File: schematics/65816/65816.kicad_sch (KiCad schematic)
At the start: 2 parts

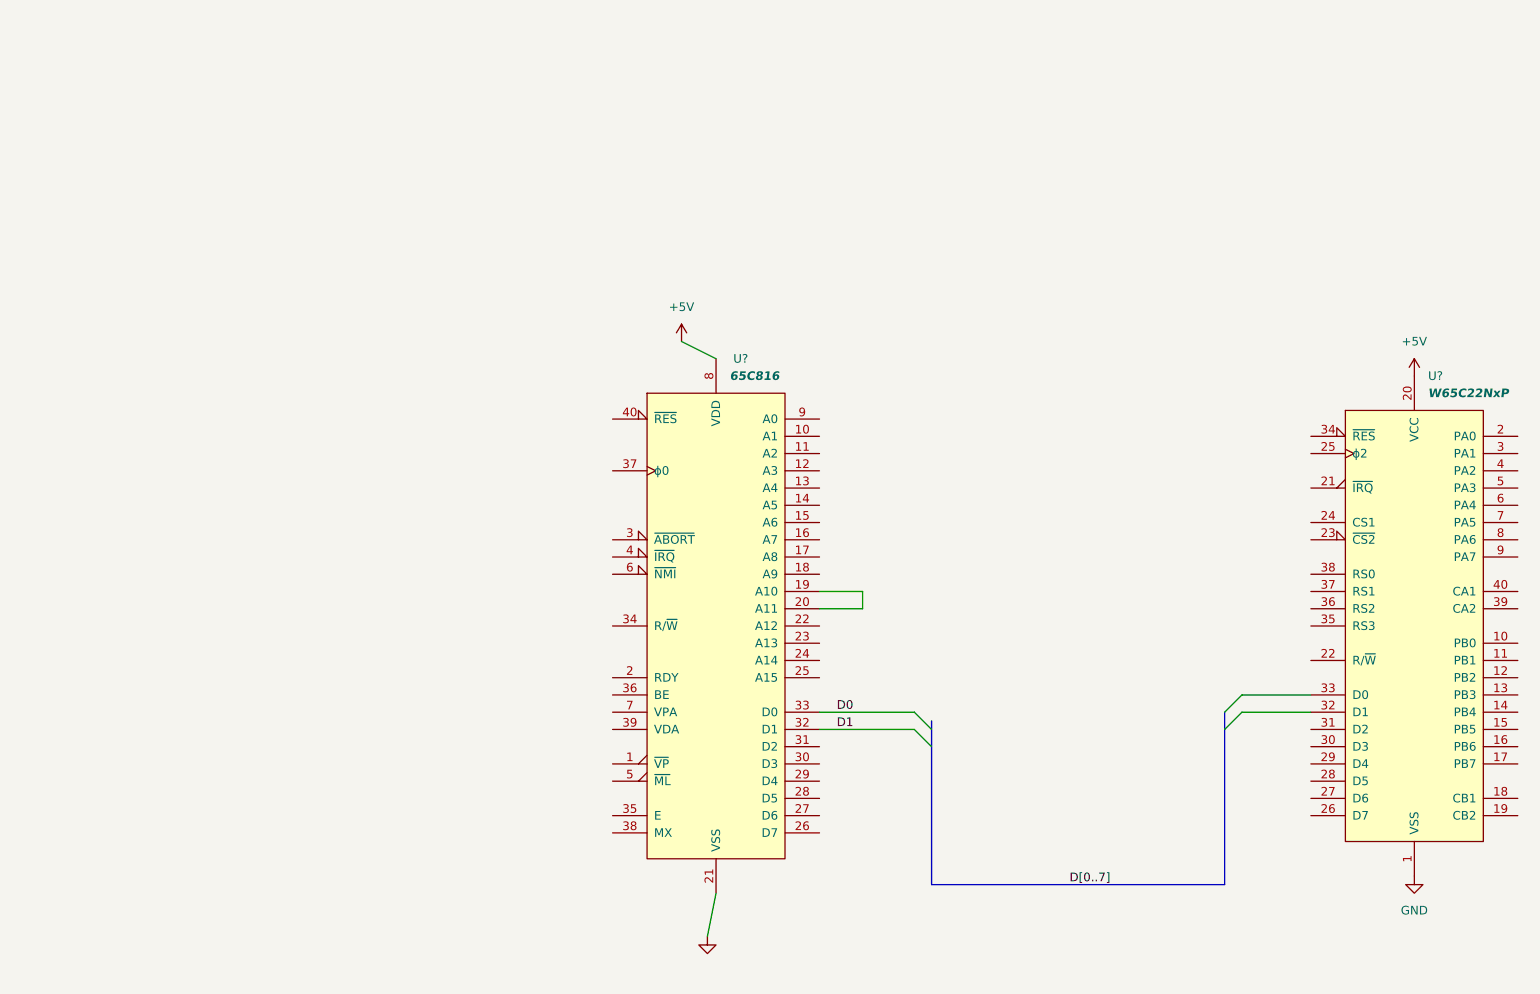
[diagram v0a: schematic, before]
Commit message: schematics
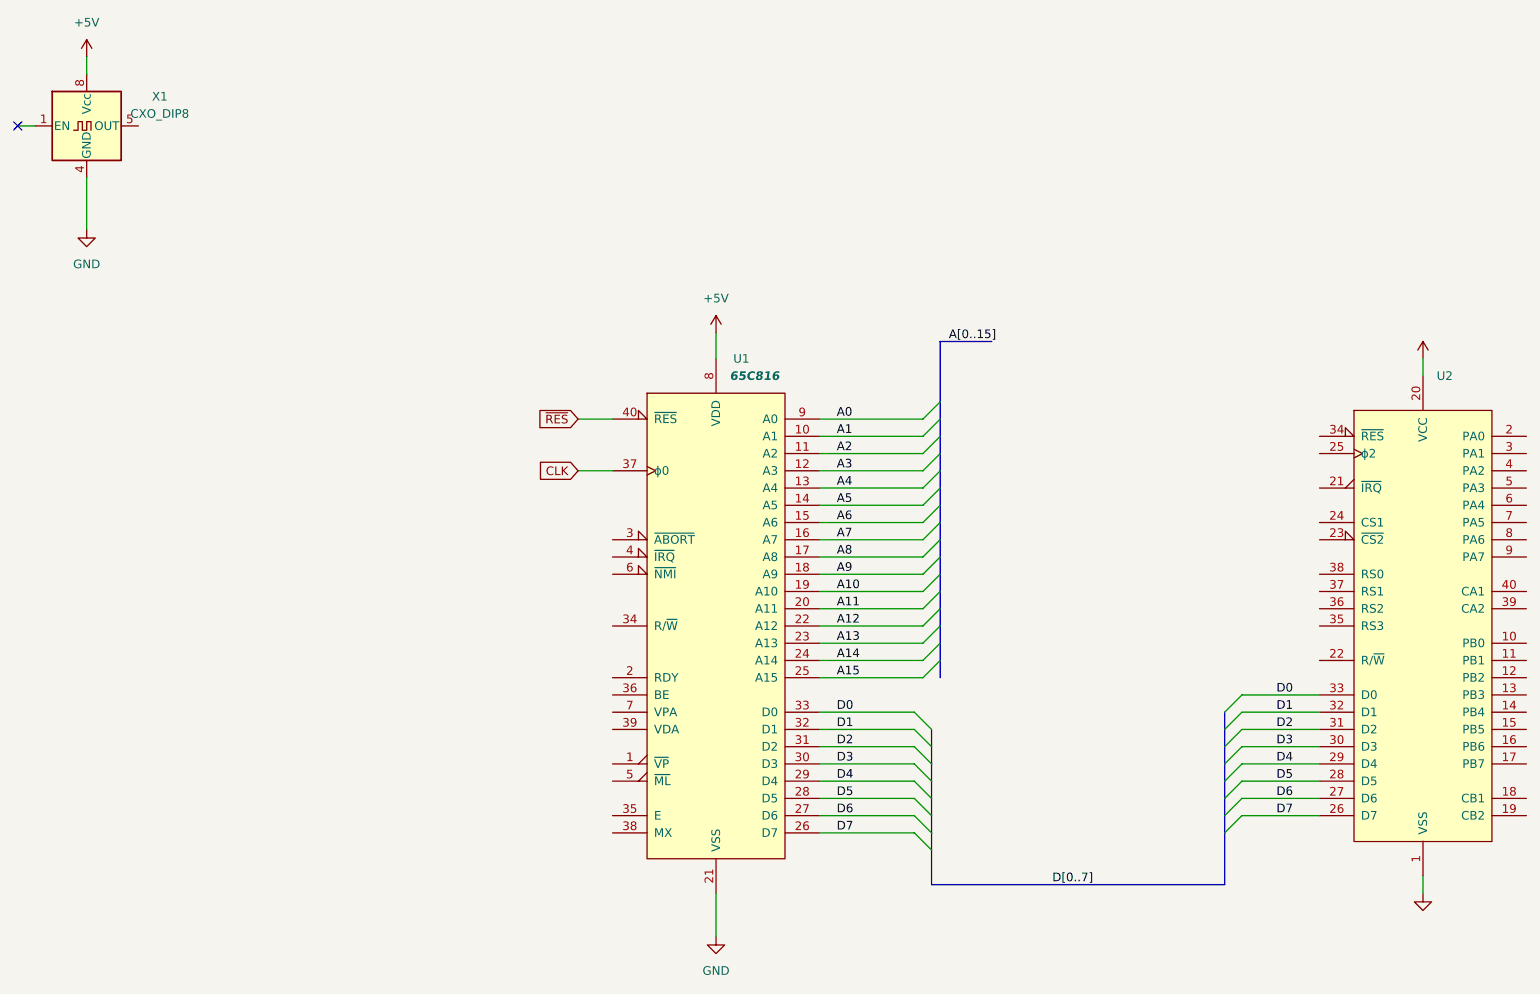
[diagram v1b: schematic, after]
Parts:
- added X1: CXO_DIP8, Oscillator:Oscillator_DIP-8, symbol Oscillator:CXO_DIP8
- U2: renamed from U?; value W65C22NxP -> (none)
- gave numbers to parts that had none: 1
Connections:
- net +5V: now also X1.8 (Vcc)
- net D0: now also U2.33 (D0)
- net D1: now also U2.32 (D1)
- net GND: now also X1.4 (GND)
- net D7: now reaches U2.26 (D7)
- net D7: now also U1.26 (D7)
- net D6: now reaches U2.27 (D6)
- net D6: now also U1.27 (D6)
- net D5: now reaches U2.28 (D5)
- net D5: now also U1.28 (D5)
- net D4: now reaches U2.29 (D4)
- net D4: now also U1.29 (D4)
- net D3: now reaches U2.30 (D3)
- net D3: now also U1.30 (D3)
- net D2: now reaches U2.31 (D2)
- net D2: now also U1.31 (D2)
- net A1: now reaches U1.10 (A1)
- net A2: now reaches U1.11 (A2)
- net A3: now reaches U1.12 (A3)
- net A4: now reaches U1.13 (A4)
- net A5: now reaches U1.14 (A5)
- net A6: now reaches U1.15 (A6)
- net A7: now reaches U1.16 (A7)
- net A8: now reaches U1.17 (A8)
- net A9: now reaches U1.18 (A9)
- net A10: now reaches U1.19 (A10)
- net A10: no longer U1.20 (A11)
- net A12: now reaches U1.22 (A12)
- net A13: now reaches U1.23 (A13)
- net A14: now reaches U1.24 (A14)
- net A15: now reaches U1.25 (A15)
- net CLK: now reaches U1.37 (ϕ0)
- net ~{RES}: now reaches U1.40 (~{RES})
- net A0: now reaches U1.9 (A0)
- new net A11: U1.20 (A11)
- no-connect marks 0 -> 1
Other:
- company: (none) -> Alexander Hansen
- title: (none) -> 65816
- moved on the sheet: U2
